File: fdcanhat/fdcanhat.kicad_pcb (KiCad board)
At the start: 2 copper layers, 65 x 56.5 mm, 9 parts, among them J1 Raspberry_Pi_5

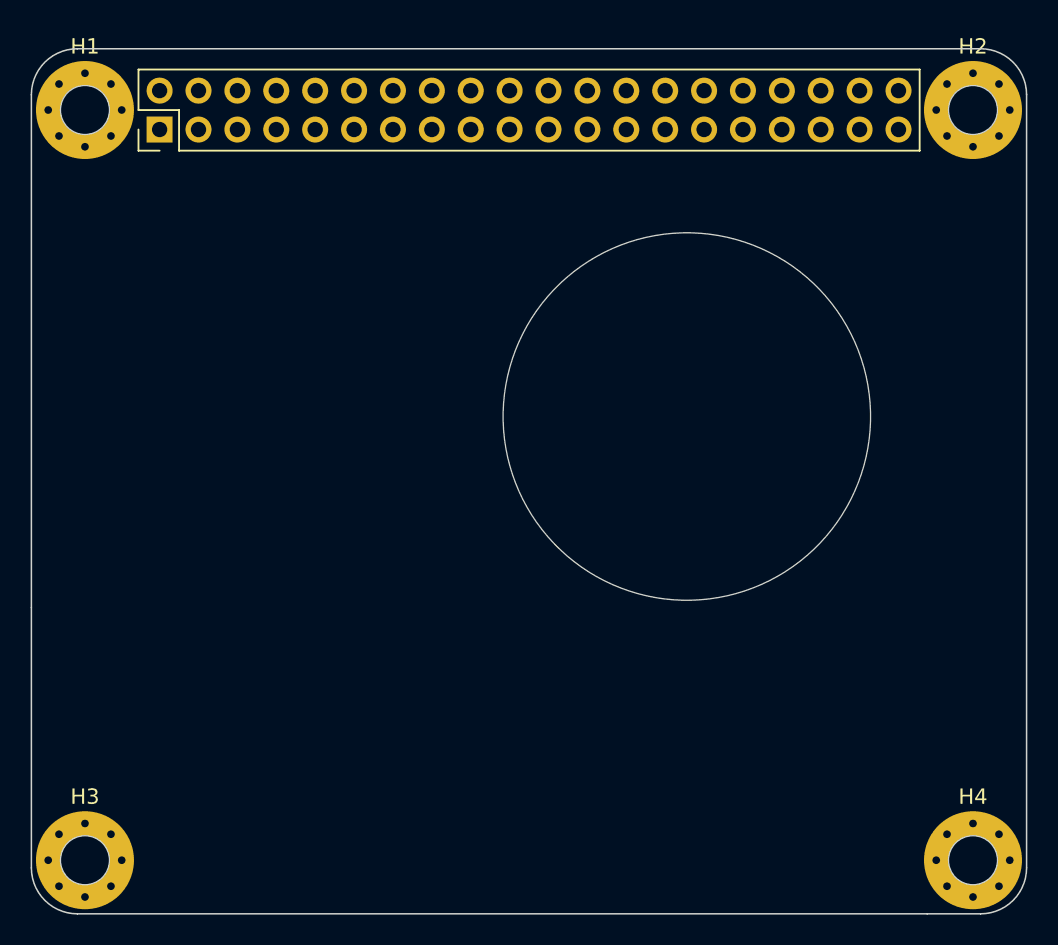
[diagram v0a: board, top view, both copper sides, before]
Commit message: almost done
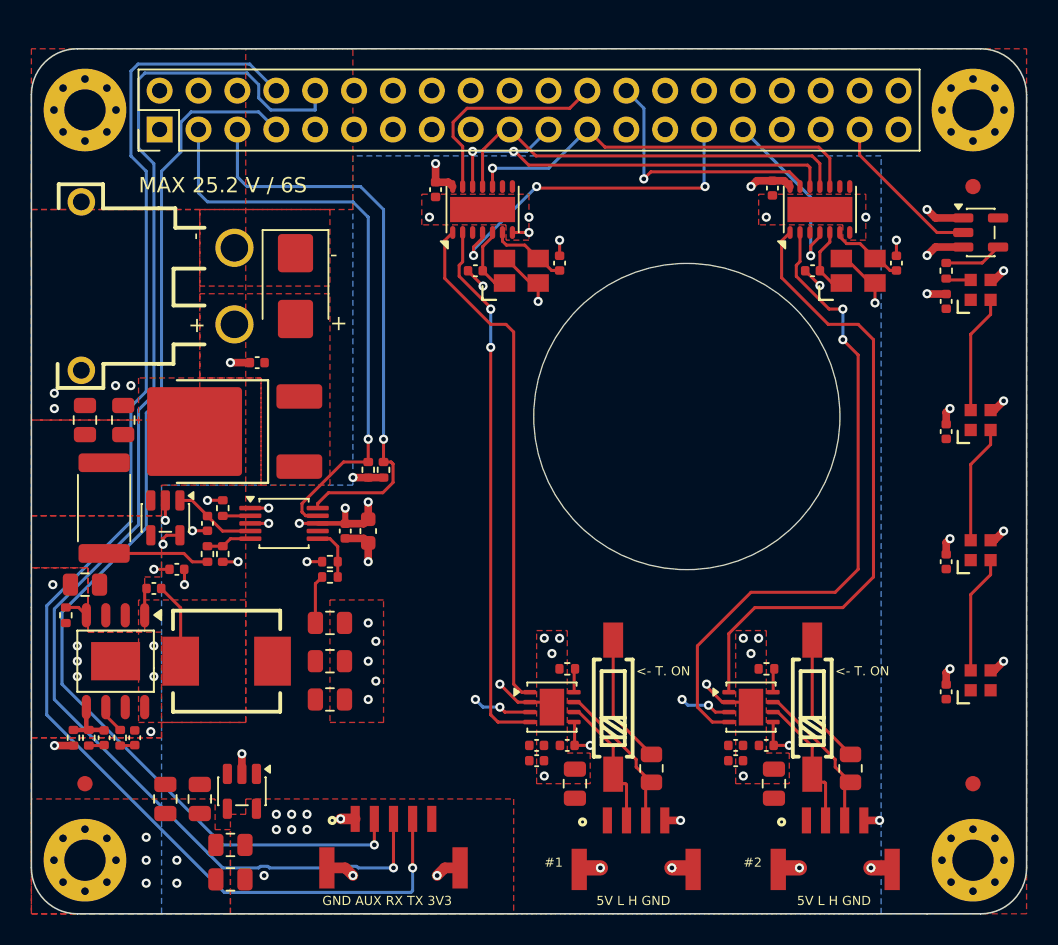
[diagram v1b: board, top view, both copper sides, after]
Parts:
- removed ? (x4): , 
- added C1: 100n 50V X7R, 0_capacitor_smd:C_0402_1005Metric, F.Cu at (124.8, 84.5)
- added C10: 22u 25V X5R, 0_capacitor_smd:C_0805_2012Metric, F.Cu at (129.5, 104.0)
- added C11: 22u 25V X5R, 0_capacitor_smd:C_0805_2012Metric, F.Cu at (129.5, 106.5)
- added C12: 2n7 50V X7R, 0_capacitor_smd:C_0402_1005Metric, F.Cu at (116.8, 109.0)
- added C13: 10u 50V X5R, 0_capacitor_smd:C_0805_2012Metric, F.Cu at (118.8, 113.0)
- added C14: 10u 50V X5R, 0_capacitor_smd:C_0805_2012Metric, F.Cu at (121.0, 113.0)
- added C15: 10u 50V X5R, 0_capacitor_smd:C_0805_2012Metric, F.Cu at (123.0, 118.2)
- added C16: 10u 50V X5R, 0_capacitor_smd:C_0805_2012Metric, F.Cu at (123.0, 116.0)
- added C17: 1u 25V X7R, 0_capacitor_smd:C_0402_1005Metric, F.Cu at (143.0, 110.5)
- added C18: 100n 50V X7R, 0_capacitor_smd:C_0402_1005Metric, F.Cu at (143.0, 109.5)
- added C19: 100n 50V X7R, 0_capacitor_smd:C_0402_1005Metric, F.Cu at (145.0, 109.5)
- added C2: 10u 50V X5R, 0_capacitor_smd:C_0805_2012Metric, F.Cu at (113.5, 88.2)
- added C20: 10u 50V X5R, 0_capacitor_smd:C_0805_2012Metric, F.Cu at (145.5, 112.0)
- added C21: 100n 50V X7R, 0_capacitor_smd:C_0402_1005Metric, F.Cu at (136.4, 73.2)
- added C22: 27p 50V C0G, 0_capacitor_smd:C_0402_1005Metric, F.Cu at (139.0, 78.5)
- added C23: 27p 50V C0G, 0_capacitor_smd:C_0402_1005Metric, F.Cu at (144.5, 78.0)
- added C24: 1u 25V X7R, 0_capacitor_smd:C_0402_1005Metric, F.Cu at (156.0, 110.5)
- added C25: 100n 50V X7R, 0_capacitor_smd:C_0402_1005Metric, F.Cu at (156.0, 109.5)
- added C26: 100n 50V X7R, 0_capacitor_smd:C_0402_1005Metric, F.Cu at (158.0, 109.5)
- added C27: 10u 50V X5R, 0_capacitor_smd:C_0805_2012Metric, F.Cu at (158.5, 112.0)
- added C28: 100n 50V X7R, 0_capacitor_smd:C_0402_1005Metric, F.Cu at (158.4, 73.1)
- added C29: 27p 50V C0G, 0_capacitor_smd:C_0402_1005Metric, F.Cu at (161.0, 78.5)
- added C3: 10u 50V X5R, 0_capacitor_smd:C_0805_2012Metric, F.Cu at (116.0, 88.2)
- added C30: 27p 50V C0G, 0_capacitor_smd:C_0402_1005Metric, F.Cu at (166.5, 78.0)
- added C31: 100n 50V X7R, 0_capacitor_smd:C_0402_1005Metric, F.Cu at (169.8, 80.5)
- added C32: 100n 50V X7R, 0_capacitor_smd:C_0402_1005Metric, F.Cu at (169.8, 97.5)
- added C33: 100n 50V X7R, 0_capacitor_smd:C_0402_1005Metric, F.Cu at (169.8, 89.0)
- added C34: 100n 50V X7R, 0_capacitor_smd:C_0402_1005Metric, F.Cu at (169.8, 106.0)
- added C35: 1u 50V X5R, 0_capacitor_smd:C_0603_1608Metric, F.Cu at (132.0, 95.5)
- added C36: 100n 50V X7R, 0_capacitor_smd:C_0402_1005Metric, F.Cu at (130.5, 95.5)
- added C4: 100n 50V X7R, 0_capacitor_smd:C_0402_1005Metric, F.Cu at (119.5, 98.0)
- added C5: 100n 50V X7R, 0_capacitor_smd:C_0402_1005Metric, F.Cu at (121.5, 95.0)
- added C6: 100n 50V X7R, 0_capacitor_smd:C_0402_1005Metric, F.Cu at (118.0, 99.2)
- added C7: 10u 50V X5R, 0_capacitor_smd:C_0805_2012Metric, F.Cu at (113.5, 99.0)
- added C8: 47p 50V C0G, 0_capacitor_smd:C_0402_1005Metric, F.Cu at (114.8, 109.0)
- added C9: 22u 25V X5R, 0_capacitor_smd:C_0805_2012Metric, F.Cu at (129.5, 101.5)
- added D1: MBR1060CS, 0_diodes:TO-252-2_L6.6-W6.1-P4.57-LS10.2-TR-CW, F.Cu at (124.1, 89.0)
- added D2: SMBJ28CA, Diode_SMD:D_SMB, F.Cu at (127.2, 79.5)
- added D3: SK6812, 0_diodes:LED-SMD_4P-L2.0-W2.0-BR, F.Cu at (172.0, 79.8)
- added D4: SK6812, 0_diodes:LED-SMD_4P-L2.0-W2.0-BR, F.Cu at (172.0, 88.2)
- added D5: SK6812, 0_diodes:LED-SMD_4P-L2.0-W2.0-BR, F.Cu at (172.0, 96.8)
- added D6: SK6812, 0_diodes:LED-SMD_4P-L2.0-W2.0-BR, F.Cu at (172.0, 105.2)
- added FID1: Fiducial, Fiducial:Fiducial_1mm_Mask2mm, F.Cu at (171.5, 112.0)
- added FID2: Fiducial, Fiducial:Fiducial_1mm_Mask2mm, F.Cu at (171.5, 73.0)
- added FID3: Fiducial, Fiducial:Fiducial_1mm_Mask2mm, F.Cu at (113.5, 112.0)
- added J2: GH1.25-5P, 0_connectors:SM05B-GHS-TB-LF-SN, F.Cu at (133.7, 115.9)
- added J3: XT30 M, 0_connectors:XT30PW-M, F.Cu at (118.3, 79.5)
- added J4: GH1.25-4P, 0_connectors:SM04B-GHS-TB-LF-SN, F.Cu at (149.5, 116.0)
- added J5: GH1.25-4P, 0_connectors:SM04B-GHS-TB-LF-SN, F.Cu at (162.5, 116.0)
- added L1: 3.3 uH @ 8.5A, 0_inductors:IND-SMD_L7.0-W6.6, F.Cu at (122.8, 104.0)
- added R1: 10m, 0_resistor_smd:R_2512_6332Metric, F.Cu at (114.8, 94.0)
- added R10: 120R, 0_resistor_smd:R_0805_2012Metric, F.Cu at (150.5, 111.0)
- added R11: 10k, 0_resistor_smd:R_0402_1005Metric, F.Cu at (145.0, 104.5)
- added R12: 120R, 0_resistor_smd:R_0805_2012Metric, F.Cu at (163.5, 111.0)
- added R13: 10k, 0_resistor_smd:R_0402_1005Metric, F.Cu at (158.0, 104.5)
- added R14: 22R, 0_resistor_smd:R_0402_1005Metric, F.Cu at (169.8, 78.5)
- added R15: 10k, 0_resistor_smd:R_0402_1005Metric, F.Cu at (122.5, 94.0)
- added R16: 10k, 0_resistor_smd:R_0402_1005Metric, F.Cu at (132.0, 91.5)
- added R17: 10k, 0_resistor_smd:R_0402_1005Metric, F.Cu at (133.0, 91.5)
- added R2: 100k, 0_resistor_smd:R_0402_1005Metric, F.Cu at (121.5, 97.0)
- added R3: 10k, 0_resistor_smd:R_0402_1005Metric, F.Cu at (122.5, 97.0)
- added R4: 33k, 0_resistor_smd:R_0402_1005Metric, F.Cu at (129.5, 98.5)
- added R5: 53k6, 0_resistor_smd:R_0402_1005Metric, F.Cu at (113.8, 109.0)
- added R6: 10k, 0_resistor_smd:R_0402_1005Metric, F.Cu at (129.5, 97.5)
- added R7: 200K, 0_resistor_smd:R_0402_1005Metric, F.Cu at (112.2, 101.0)
- added R8: 15k8, 0_resistor_smd:R_0402_1005Metric, F.Cu at (115.8, 109.0)
- added R9: 10k, 0_resistor_smd:R_0402_1005Metric, F.Cu at (112.8, 109.0)
- added SW1: SW_SPST, 0_misc:SW-SMD_DSIC01LSGET, F.Cu at (148.0, 107.0)
- added SW2: SW_SPST, 0_misc:SW-SMD_DSIC01LSGET, F.Cu at (161.0, 107.0)
- added U1: INA180, 0_transceivers:SOT-23-5, F.Cu at (118.8, 94.6)
- added U2: AP64500, 0_power:SO-8-EP, F.Cu at (115.5, 104.0)
- added U3: SPX3819, 0_power:SOT-23-5, F.Cu at (123.8, 112.5)
- added U4: TJA1051TK-3, 0_transceivers:HVSON-8-1EP_3x3mm_P0.65mm_EP1.6x2.4mm, F.Cu at (144.0, 107.0)
- added U5: MCP2518FDT, 0_transceivers:DFN-14-1EP_3x4.5mm_P0.65mm_EP1.65x4.25mm, F.Cu at (139.5, 74.5)
- added U6: TJA1051TK-3, 0_transceivers:HVSON-8-1EP_3x3mm_P0.65mm_EP1.6x2.4mm, F.Cu at (157.0, 107.0)
- added U7: MCP2518FDT, 0_transceivers:DFN-14-1EP_3x4.5mm_P0.65mm_EP1.65x4.25mm, F.Cu at (161.5, 74.5)
- added U8: 74AHCT1G125, 0_transceivers:SOT-23-5, F.Cu at (172.0, 76.0)
- added U9: ADS1115IDGSR, 0_transceivers:VSSOP-10_3x3mm_P0.5mm, F.Cu at (126.5, 95.0)
- added Y1: 20 MHz, 0_misc:CRYSTAL-SMD_4P-L3.2-W2.5-BL-2, F.Cu at (142.0, 78.5)
- added Y2: 20 MHz, 0_misc:CRYSTAL-SMD_4P-L3.2-W2.5-BL-2, F.Cu at (164.0, 78.5)
- H1, H2, H3, H4: footprint 0_misc:MountingHole_3.2mm_M3_Pad_Via -> MountingHole:MountingHole_2.7mm_M2.5_Pad_Via
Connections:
- J1 pad 15: /RTK_PPS -> unconnected-(J1-GPIO22/SDIO_CLK-Pad15)
- J1 pad 16: /RTK_EVENT -> unconnected-(J1-GPIO23/SDIO_CMD-Pad16)
- J1 pad 19: /SPI0_MOSI -> /FDCAN/SPI0_MOSI
- J1 pad 21: /SPI0_MISO -> /FDCAN/SPI0_MISO
- J1 pad 23: /SPI0_SCK -> /FDCAN/SPI0_SCK
- J1 pad 32: /ADD_LED -> unconnected-(J1-GPIO12/PWM0-Pad32)
- J1 pad 33: /BUZZER -> unconnected-(J1-GPIO13/PWM1-Pad33)
- J1 pad 37: unconnected-(J1-GPIO26/SDIO_DAT2-Pad37) -> /ADD_LED
- J1 pad 7: unconnected-(J1-GPCLK0/GPIO04-Pad7) -> /RTK_PPS
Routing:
- net /RTK_TXD: track 0.00 -> 89.0 mm, vias 0 -> 1
- net /RTK_RXD: track 0.00 -> 88.7 mm, vias 0 -> 1
- net /RTK_PPS: track 0.00 -> 73.4 mm, vias 0 -> 1
- net GND: track 0.00 -> 62.4 mm, vias 0 -> 72
- net /FDCAN/FDCAN2_RX: track 0.00 -> 43.3 mm, vias 0 -> 2
- net /FDCAN/FDCAN2_TX: track 0.00 -> 41.2 mm
- net /MON_SDA: track 0.00 -> 39.0 mm, vias 0 -> 1
- net /MON_SCL: track 0.00 -> 37.7 mm, vias 0 -> 1
- net /FDCAN/FDCAN1_RX: track 0.00 -> 35.2 mm, vias 0 -> 2
- net /FDCAN/FDCAN1_TX: track 0.00 -> 33.4 mm
- net /FDCAN/SPI0_MISO: track 0.00 -> 28.9 mm, vias 0 -> 2
- net /FDCAN/SPI0_MOSI: track 0.00 -> 27.4 mm
- net /FDCAN/SPI0_SCK: track 0.00 -> 26.9 mm, vias 0 -> 1
- net /FDCAN1_INT: track 0.00 -> 22.8 mm, vias 0 -> 3
- net +3V3: track 0.00 -> 22.8 mm, vias 0 -> 18
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- added copper zone on B.Cu, net +3V3
- added copper zone on F.Cu, net +3V3
- added copper zone on F.Cu, net +5V
- added copper zone on F.Cu, net +BAT
- added copper zone on F.Cu, net +BAT_PROT
- added copper zone on F.Cu, net +BAT_PROT_PRE_MEAS
- added copper zone on F.Cu, net /Power Generation/BUCK_SW
- added copper zone on F.Cu, net GND
- added copper zone on In1.Cu, net GND
- added copper zone on In2.Cu, net GND
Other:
- outline, holes or cut-outs redrawn
- copper layers 2 -> 4
- board text added: "#1"
- board text added: "#2"
- board text added: "+"
- board text added: "-"
- board text added: "5V L H GND"
- board text added: "<- T. ON"
- board text added: "GND AUX RX TX 3V3"
- board text added: "MAX 25.2 V / 6S"
